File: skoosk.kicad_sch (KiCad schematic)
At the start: 2 parts

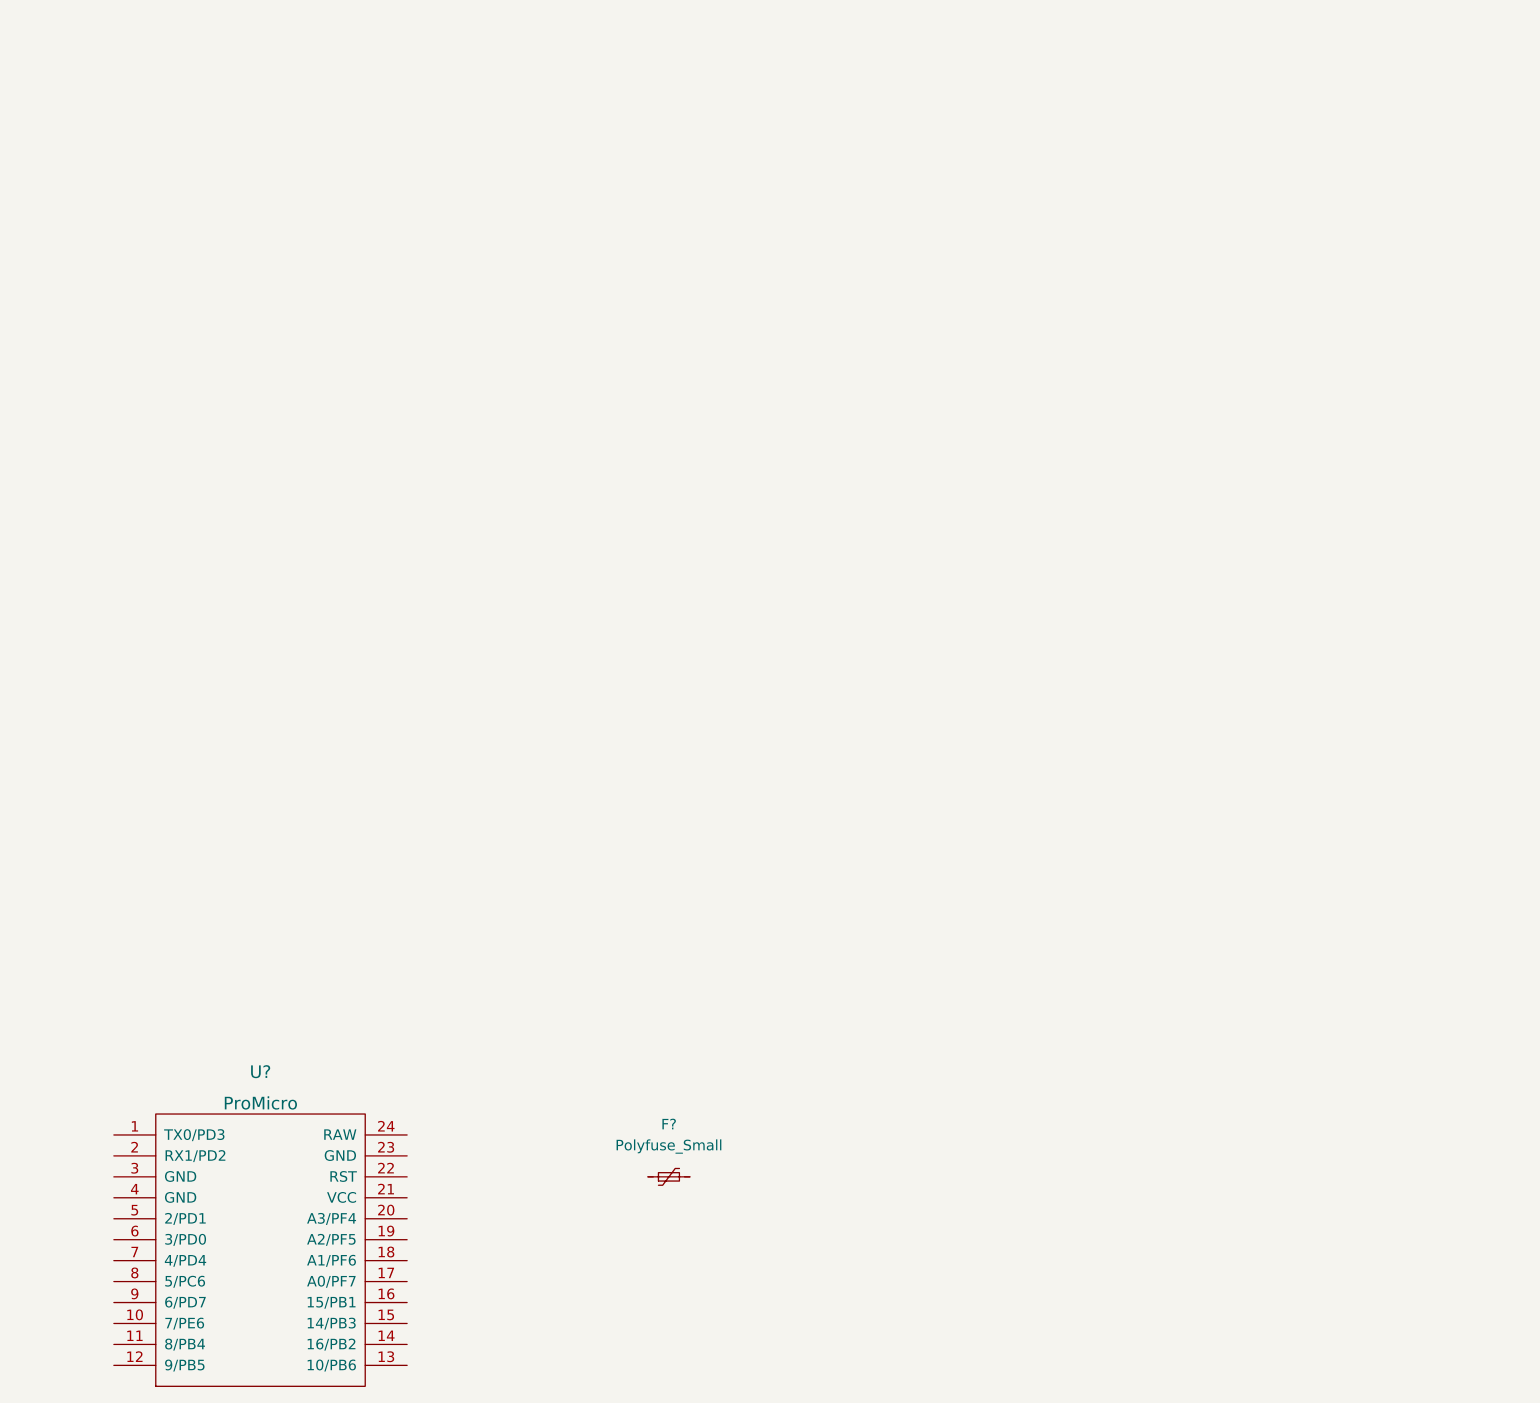
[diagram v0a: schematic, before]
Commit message: switch matrix build, footprints layed out
missing is MCU footprint, reset switch, traces

do i want underglow?
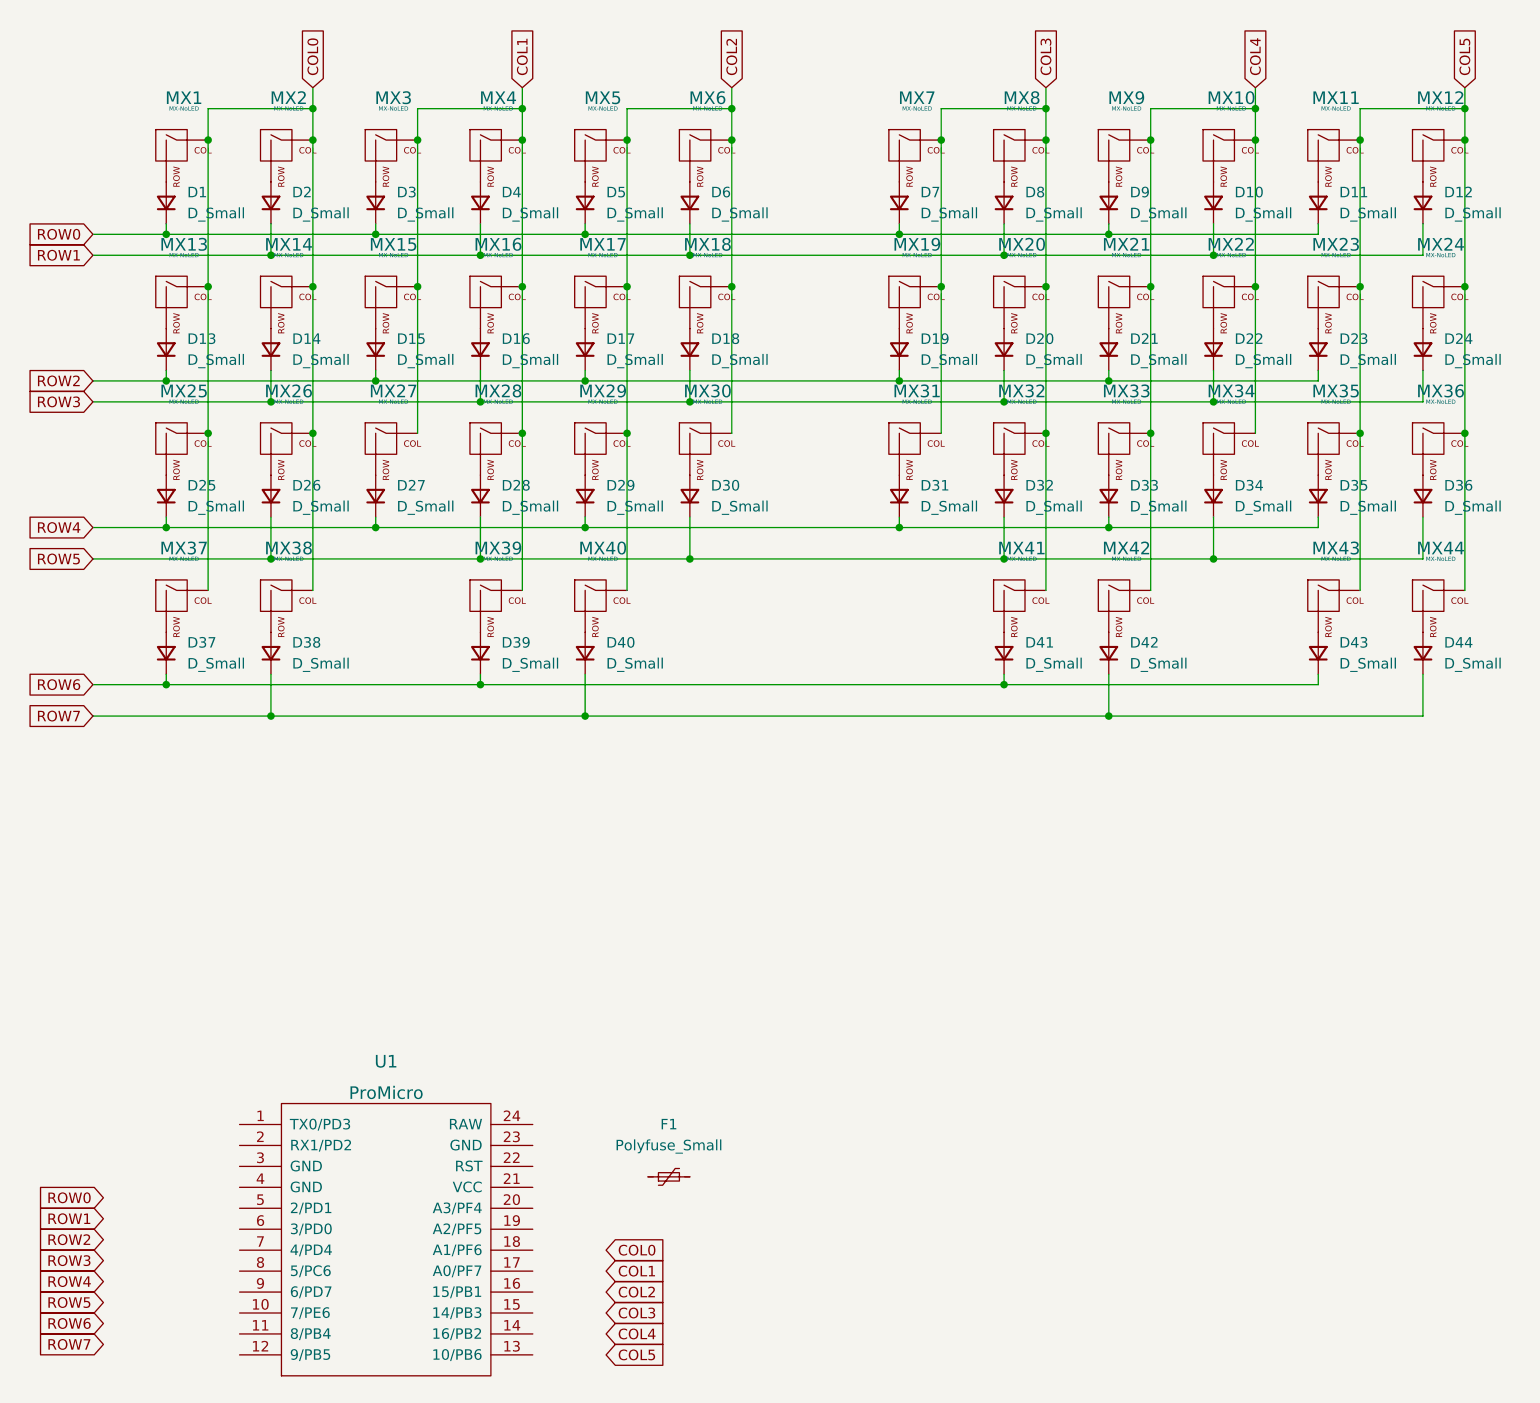
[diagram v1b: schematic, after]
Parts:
- added D1, D10, D11, D12, D13, D14, D15, D16, D17, D18, D19, D2, D20, D21, D22, D23, D24, D25, D26, D27, D28, D29, D3, D30, D31, D32, D33, D34, D35, D36, D37, D38, D39, D4, D40, D41, D42, D43, D44, D5, D6, D7, D8, D9: D_Small, symbol Device:D_Small
- added MX1, MX12, MX13, MX24, MX25, MX36, MX37, MX38, MX39, MX42, MX43, MX44: MX-NoLED, MX_Only:MXOnly-1.25U-NoLED, symbol MX_Alps_Hybrid:MX-NoLED
- added MX10, MX11, MX14, MX15, MX16, MX17, MX18, MX19, MX2, MX20, MX21, MX22, MX23, MX26, MX27, MX28, MX29, MX3, MX30, MX31, MX32, MX33, MX34, MX35, MX4, MX5, MX6, MX7, MX8, MX9: MX-NoLED, MX_Only:MXOnly-1U-NoLED, symbol MX_Alps_Hybrid:MX-NoLED
- added MX40, MX41: MX-NoLED, MX_Only:MXOnly-3U-NoLED, symbol MX_Alps_Hybrid:MX-NoLED
- gave numbers to parts that had none: 2
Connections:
- new net: D25.2 (A), MX25.2 (ROW)
- new net: D16.2 (A), MX16.2 (ROW)
- new net: D43.2 (A), MX43.2 (ROW)
- new net: D9.2 (A), MX9.2 (ROW)
- new net: D24.2 (A), MX24.2 (ROW)
- new net: D1.2 (A), MX1.2 (ROW)
- new net: D21.2 (A), MX21.2 (ROW)
- new net: D12.2 (A), MX12.2 (ROW)
- new net: D17.2 (A), MX17.2 (ROW)
- new net: D23.2 (A), MX23.2 (ROW)
- new net: D42.2 (A), MX42.2 (ROW)
- new net: D4.2 (A), MX4.2 (ROW)
- new net: D8.2 (A), MX8.2 (ROW)
- new net: D3.2 (A), MX3.2 (ROW)
- new net: D26.2 (A), MX26.2 (ROW)
- new net: D44.2 (A), MX44.2 (ROW)
- new net: D5.2 (A), MX5.2 (ROW)
- new net: D2.2 (A), MX2.2 (ROW)
- new net: D10.2 (A), MX10.2 (ROW)
- new net: D11.2 (A), MX11.2 (ROW)
- new net: D33.2 (A), MX33.2 (ROW)
- new net: D20.2 (A), MX20.2 (ROW)
- new net: D29.2 (A), MX29.2 (ROW)
- new net: D27.2 (A), MX27.2 (ROW)
- new net: D28.2 (A), MX28.2 (ROW)
- new net: D35.2 (A), MX35.2 (ROW)
- new net: D7.2 (A), MX7.2 (ROW)
- new net: D30.2 (A), MX30.2 (ROW)
- new net: D38.2 (A), MX38.2 (ROW)
- new net: D19.2 (A), MX19.2 (ROW)
- new net: D41.2 (A), MX41.2 (ROW)
- new net: D37.2 (A), MX37.2 (ROW)
- new net: D15.2 (A), MX15.2 (ROW)
- new net: D14.2 (A), MX14.2 (ROW)
- new net: D31.2 (A), MX31.2 (ROW)
- new net: D13.2 (A), MX13.2 (ROW)
- new net: D18.2 (A), MX18.2 (ROW)
- new net: D34.2 (A), MX34.2 (ROW)
- new net: D22.2 (A), MX22.2 (ROW)
- new net: D6.2 (A), MX6.2 (ROW)
- new net: D36.2 (A), MX36.2 (ROW)
- new net: D40.2 (A), MX40.2 (ROW)
- new net: D39.2 (A), MX39.2 (ROW)
- new net: D32.2 (A), MX32.2 (ROW)
- new net COL0: MX1.1 (COL), MX13.1 (COL), MX14.1 (COL), MX2.1 (COL), MX25.1 (COL), MX26.1 (COL), MX37.1 (COL), MX38.1 (COL)
- new net COL1: MX15.1 (COL), MX16.1 (COL), MX27.1 (COL), MX28.1 (COL), MX3.1 (COL), MX39.1 (COL), MX4.1 (COL)
- new net COL2: MX17.1 (COL), MX18.1 (COL), MX29.1 (COL), MX30.1 (COL), MX40.1 (COL), MX5.1 (COL), MX6.1 (COL)
- new net COL3: MX19.1 (COL), MX20.1 (COL), MX31.1 (COL), MX32.1 (COL), MX41.1 (COL), MX7.1 (COL), MX8.1 (COL)
- new net COL4: MX10.1 (COL), MX21.1 (COL), MX22.1 (COL), MX33.1 (COL), MX34.1 (COL), MX42.1 (COL), MX9.1 (COL)
- new net COL5: MX11.1 (COL), MX12.1 (COL), MX23.1 (COL), MX24.1 (COL), MX35.1 (COL), MX36.1 (COL), MX43.1 (COL), MX44.1 (COL)
- new net ROW0: D1.1 (K), D11.1 (K), D3.1 (K), D5.1 (K), D7.1 (K), D9.1 (K)
- new net ROW1: D10.1 (K), D12.1 (K), D2.1 (K), D4.1 (K), D6.1 (K), D8.1 (K)
- new net ROW2: D13.1 (K), D15.1 (K), D17.1 (K), D19.1 (K), D21.1 (K), D23.1 (K)
- new net ROW3: D14.1 (K), D16.1 (K), D18.1 (K), D20.1 (K), D22.1 (K), D24.1 (K)
- new net ROW4: D25.1 (K), D27.1 (K), D29.1 (K), D31.1 (K), D33.1 (K), D35.1 (K)
- new net ROW5: D26.1 (K), D28.1 (K), D30.1 (K), D32.1 (K), D34.1 (K), D36.1 (K)
- new net ROW6: D37.1 (K), D39.1 (K), D41.1 (K), D43.1 (K)
- new net ROW7: D38.1 (K), D40.1 (K), D42.1 (K), D44.1 (K)
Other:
- moved on the sheet: U1
